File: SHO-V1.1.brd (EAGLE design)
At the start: 25.1 x 26 mm, 16 parts, among them Q1 BS170

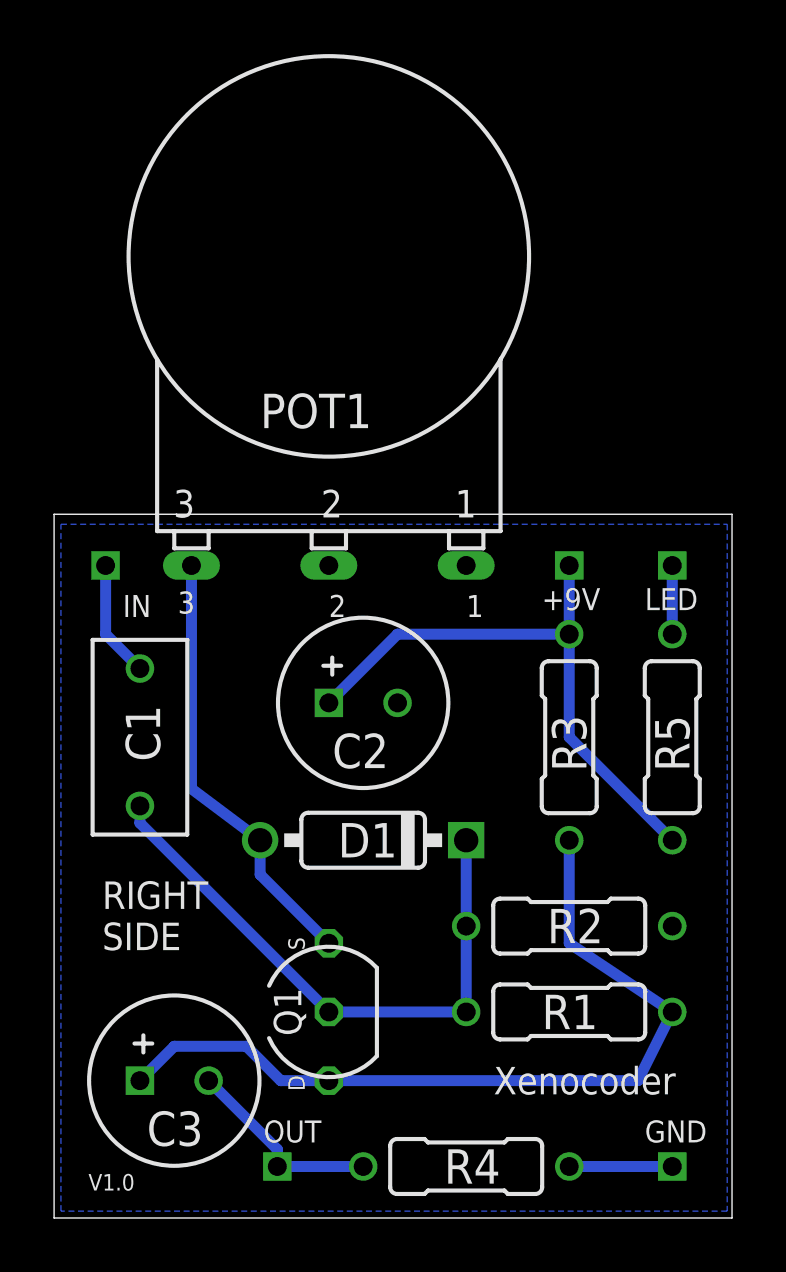
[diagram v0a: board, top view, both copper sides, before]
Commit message: New schematic and Board layout
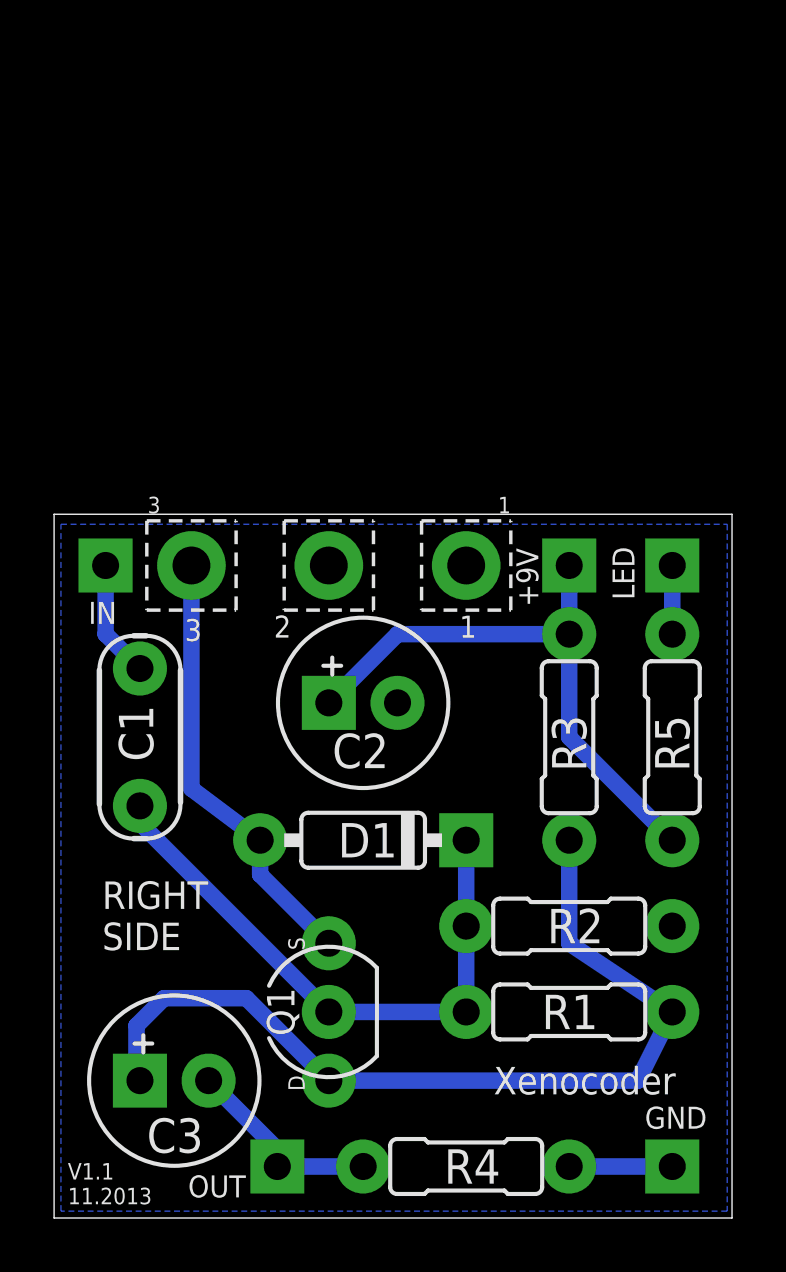
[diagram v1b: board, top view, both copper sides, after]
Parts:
- +9V, GND, IN, LED, OUT: device gm-supply:SQUARE -> mb_supply:SQUARE
- C1: device gm-caps-film-box:072X035 -> mb_caps-chicklet:075X030
- C2, C3: device gm-caps-electro-pol:063_025 -> mb_caps-electro:063_025
- D1: device gm-diodes:DO35-3 -> mb_diodes:DO35-3
- POT1: device gm-pots:16MM -> mb_pots:16MM_PCB_PADS
- Q1: device gm-trans:SOT54ES -> mb_trans:SOT54ES
- R1, R2, R3, R4, R5: device gm-resistors:R0207/3 -> mb_resistors:R0207/3
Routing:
- net N$1: track 30.7 -> 33.5 mm
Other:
- board text added: "V1.1 11.2013"
- board text removed: "V1.0"
